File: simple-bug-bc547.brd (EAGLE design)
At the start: 30.5 x 20.3 mm, 13 parts, among them T1 2N918

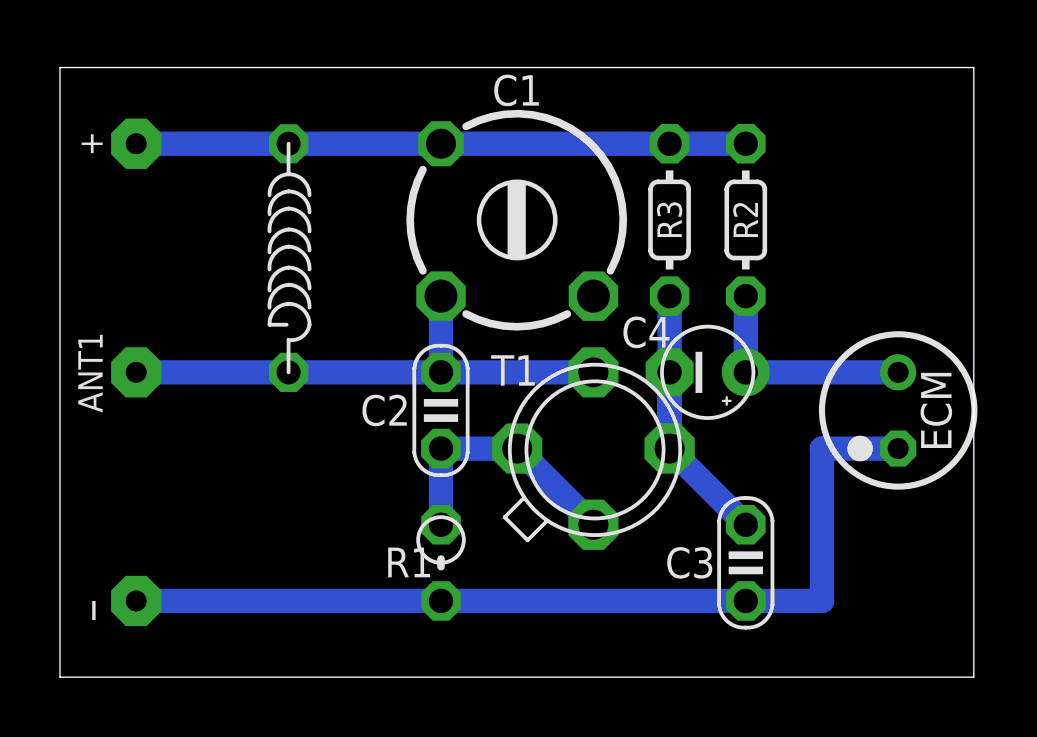
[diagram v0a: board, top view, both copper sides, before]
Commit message: ...
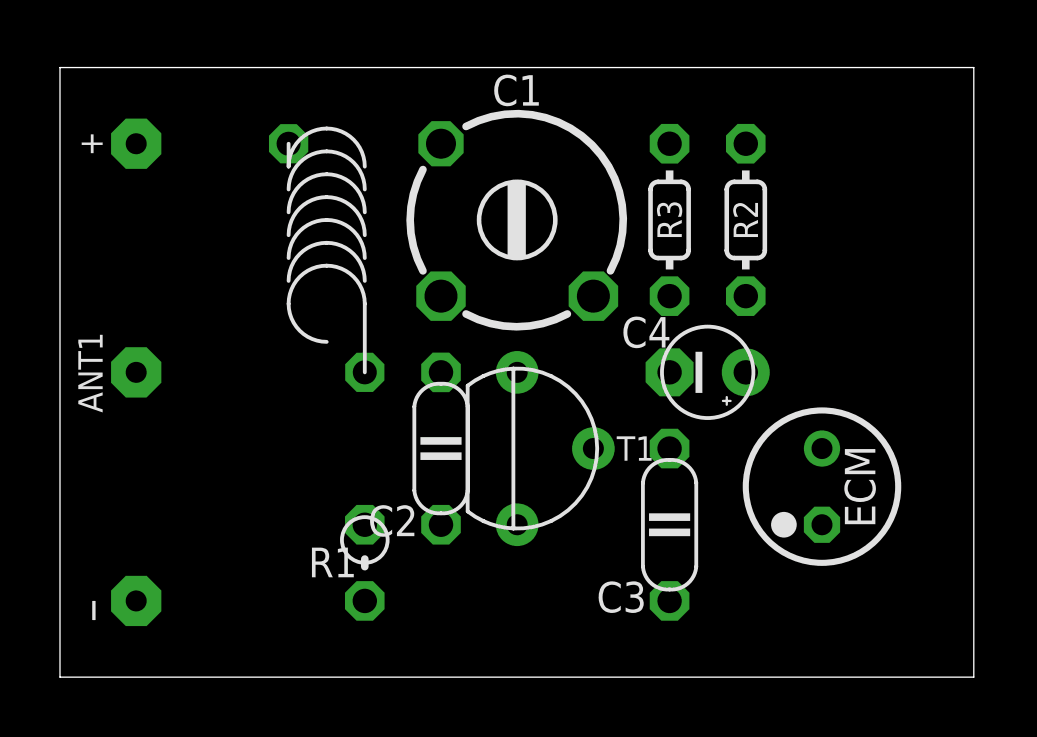
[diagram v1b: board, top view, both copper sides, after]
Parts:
- C2, C3: device c:C025-020X036 -> c:C050-020X036
- L1: device r:L-02/7 -> r:L-04/7
- T1: value 2N918 -> BC547; device 2n918:TO-72-A45 -> t:TO92-CBE-A
- moved ECM 3.59 mm to (25.4, 6.35)
- moved C3 2.84 mm to (20.3, 5.08)
- moved T1 2.54 mm to (15.2, 7.62), turned to 180 degrees
- moved R1 2.54 mm to (10.2, 3.81)
- moved C2 1.27 mm to (12.7, 7.62)
- moved L1 1.27 mm to (8.89, 14.0)
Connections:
- net N$1: now also T1.C; no longer T1.3
- net N$3: now also T1.E; no longer T1.1, T1.4
- net N$5: now also T1.B; no longer T1.2
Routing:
- net GND: track 30.5 -> 0.00 mm
- net +UB: track 20.3 -> 0.00 mm
- net N$1: track 17.8 -> 0.00 mm
- net N$5: track 11.2 -> 0.00 mm
- net N$3: track 8.67 -> 0.00 mm
- net N$6: track 7.62 -> 0.00 mm
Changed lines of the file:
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@@
 </autorouter>
 <elements>
-<element name="C2" library="c" package="C025-020X036" value="4.7pF" x="12.7" y="8.89"/>
-<element name="C3" library="c" package="C025-020X036" value="1nF" x="22.86" y="3.81"/>
-<element name="L1" library="r" package="L-02/7" value="1uH" x="7.62" y="13.97"/>
+<element name="C2" library="c" package="C050-020X036" value="4.7pF" x="12.7" y="7.62"/>
+<element name="C3" library="c" package="C050-020X036" value="1nF" x="20.32" y="5.08"/>
+<element name="L1" library="r" package="L-04/7" value="1uH" x="8.89" y="13.97"/>
 <element name="R2" library="r" package="0202/5" value="22k" x="22.86" y="15.24"/>
 <element name="R3" library="r" package="0202/5" value="47k" x="20.32" y="15.24"/>
-<element name="T1" library="2n918" package="TO-72-A45" value="2N918" x="17.78" y="7.62"/>
-<element name="ECM" library="ECM" package="ECM-5" value="ECM-5" x="27.94" y="8.89" rot="R180"/>
+<element name="T1" library="t" package="TO92-CBE-A" value="BC547" x="15.24" y="7.62" rot="R180"/>
+<element name="ECM" library="ECM" package="ECM-5" value="ECM-5" x="25.4" y="6.35" rot="R180"/>
 <element name="C1" library="cap-trim" package="TRIM808-45" value="C-TR-PH20127-45-2P23" x="15.24" y="15.24"/>
-<element name="R1" library="r" package="0202V" value="" x="12.7" y="3.81"/>
+<element name="R1" library="r" package="0202V" value="" x="10.16" y="3.81"/>
 <element name="C4" library="c" package="E2,5-3" value="" x="21.59" y="10.16"/>
 <element name="+" library="pad" package="SPAD" value="SPAD" x="2.54" y="17.78" rot="R180"/>
@@
 <signal name="N$1">
 <contactref element="L1" pad="2"/>
-<contactref element="T1" pad="3"/>
+<contactref element="T1" pad="C"/>
 <contactref element="C2" pad="1"/>
 <contactref element="C1" pad="2"/>
-<wire x1="12.7" y1="10.16" x2="17.78" y2="10.16" width="0.8128" layer="16"/>
-<wire x1="7.62" y1="10.16" x2="12.7" y2="10.16" width="0.8128" layer="16"/>
-<wire x1="12.7" y1="10.16" x2="12.7" y2="12.7" width="0.8128" layer="16"/>
 <contactref element="ANT1" pad="P"/>
-<wire x1="7.62" y1="10.16" x2="2.54" y2="10.16" width="0.8128" layer="16"/>
+<wire x1="12.7" y1="10.16" x2="15.24" y2="10.16" width="0" layer="19" extent="1-1"/>
+<wire x1="12.7" y1="12.7" x2="12.7" y2="10.16" width="0" layer="19" extent="1-1"/>
+<wire x1="10.16" y1="10.16" x2="12.7" y2="10.16" width="0" layer="19" extent="1-1"/>
+<wire x1="2.54" y1="10.16" x2="10.16" y2="10.16" width="0" layer="19" extent="1-1"/>
 </signal>
 <signal name="N$3">
 <contactref element="C2" pad="2"/>
-<contactref element="T1" pad="1"/>
-<contactref element="T1" pad="4"/>
+<contactref element="T1" pad="E"/>
 <contactref element="R1" pad="2"/>
-<wire x1="12.7" y1="5.08" x2="12.7" y2="7.62" width="0.8128" layer="16"/>
-<wire x1="15.24" y1="7.62" x2="12.7" y2="7.62" width="0.8128" layer="16"/>
-<wire x1="15.24" y1="7.62" x2="17.78" y2="5.08" width="0.8128" layer="16"/>
+<wire x1="15.24" y1="5.08" x2="10.16" y2="5.08" width="0" layer="19" extent="1-1"/>
+<wire x1="12.7" y1="5.08" x2="15.24" y2="5.08" width="0" layer="19" extent="1-1"/>
 </signal>
 <signal name="N$5">
 <contactref element="R3" pad="1"/>
 <contactref element="C3" pad="1"/>
-<contactref element="T1" pad="2"/>
+<contactref element="T1" pad="B"/>
 <contactref element="C4" pad="-"/>
-<wire x1="20.32" y1="7.62" x2="20.32" y2="12.7" width="0.8128" layer="16"/>
-<wire x1="22.86" y1="5.08" x2="20.32" y2="7.62" width="0.8128" layer="16"/>
-<wire x1="20.32" y1="7.62" x2="20.32" y2="10.16" width="0.8128" layer="16"/>
+<wire x1="20.32" y1="10.16" x2="20.32" y2="12.7" width="0" layer="19" extent="1-1"/>
+<wire x1="20.32" y1="7.62" x2="20.32" y2="10.16" width="0" layer="19" extent="1-1"/>
+<wire x1="17.78" y1="7.62" x2="20.32" y2="7.62" width="0" layer="19" extent="1-1"/>
 </signal>
 <signal name="N$6">
@@
 <contactref element="ECM" pad="2"/>
 <contactref element="C4" pad="+"/>
-<wire x1="22.86" y1="10.16" x2="27.94" y2="10.16" width="0.8128" layer="16"/>
-<wire x1="22.86" y1="10.16" x2="22.86" y2="12.7" width="0.8128" layer="16"/>
+<wire x1="22.86" y1="10.16" x2="22.86" y2="12.7" width="0" layer="19" extent="1-1"/>
+<wire x1="25.4" y1="7.62" x2="22.86" y2="10.16" width="0" layer="19" extent="1-1"/>
 </signal>
 <signal name="GND">
@@
 <contactref element="ECM" pad="1"/>
 <contactref element="R1" pad="1"/>
-<wire x1="22.86" y1="2.54" x2="25.4" y2="2.54" width="0.8128" layer="16"/>
-<wire x1="25.4" y1="2.54" x2="25.4" y2="7.62" width="0.8128" layer="16"/>
-<wire x1="25.4" y1="7.62" x2="27.94" y2="7.62" width="0.8128" layer="16"/>
-<wire x1="22.86" y1="2.54" x2="12.7" y2="2.54" width="0.8128" layer="16"/>
 <contactref element="̶̶" pad="P"/>
-<wire x1="12.7" y1="2.54" x2="2.54" y2="2.54" width="0.8128" layer="16"/>
+<wire x1="20.32" y1="2.54" x2="25.4" y2="5.08" width="0" layer="19" extent="1-1"/>
+<wire x1="10.16" y1="2.54" x2="20.32" y2="2.54" width="0" layer="19" extent="1-1"/>
+<wire x1="2.54" y1="2.54" x2="10.16" y2="2.54" width="0" layer="19" extent="1-1"/>
 </signal>
 <signal name="+UB">
@@
 <contactref element="R2" pad="2"/>
 <contactref element="C1" pad="3"/>
-<wire x1="22.86" y1="17.78" x2="20.32" y2="17.78" width="0.8128" layer="16"/>
-<wire x1="7.62" y1="17.78" x2="12.7" y2="17.78" width="0.8128" layer="16"/>
-<wire x1="12.7" y1="17.78" x2="20.32" y2="17.78" width="0.8128" layer="16"/>
 <contactref element="+" pad="P"/>
-<wire x1="7.62" y1="17.78" x2="2.54" y2="17.78" width="0.8128" layer="16"/>
+<wire x1="20.32" y1="17.78" x2="22.86" y2="17.78" width="0" layer="19" extent="1-1"/>
+<wire x1="12.7" y1="17.78" x2="20.32" y2="17.78" width="0" layer="19" extent="1-1"/>
+<wire x1="7.62" y1="17.78" x2="12.7" y2="17.78" width="0" layer="19" extent="1-1"/>
+<wire x1="2.54" y1="17.78" x2="7.62" y2="17.78" width="0" layer="19" extent="1-1"/>
 </signal>
 </signals>
